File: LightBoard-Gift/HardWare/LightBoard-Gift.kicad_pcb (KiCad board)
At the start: 2 copper layers, 87.4 x 59.4 mm, 12 parts, among them SW1 SW_Push

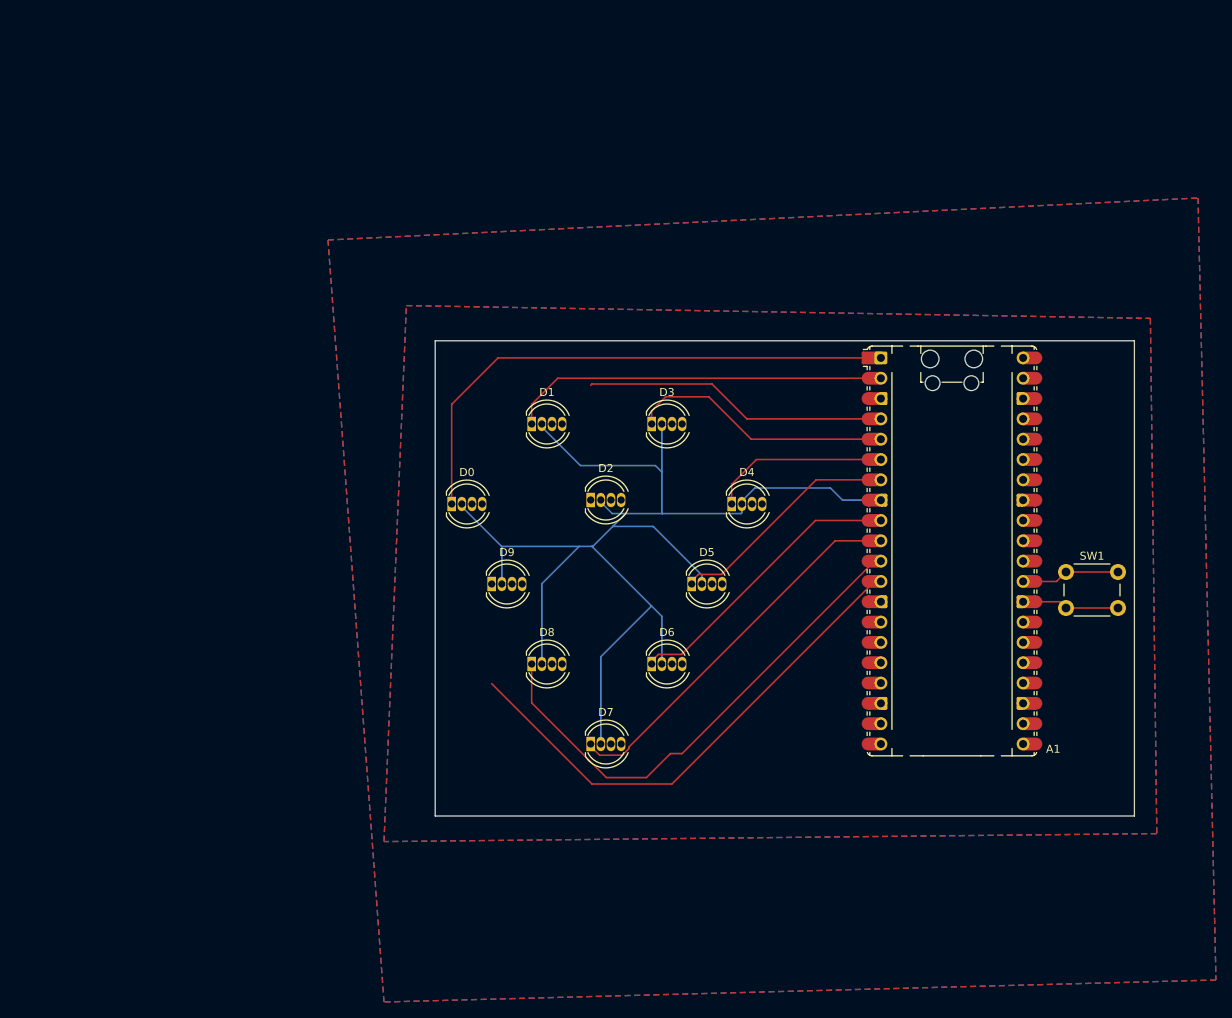
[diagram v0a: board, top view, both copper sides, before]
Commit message: Lowkey?
Forgot to save the files before pushing the last commit
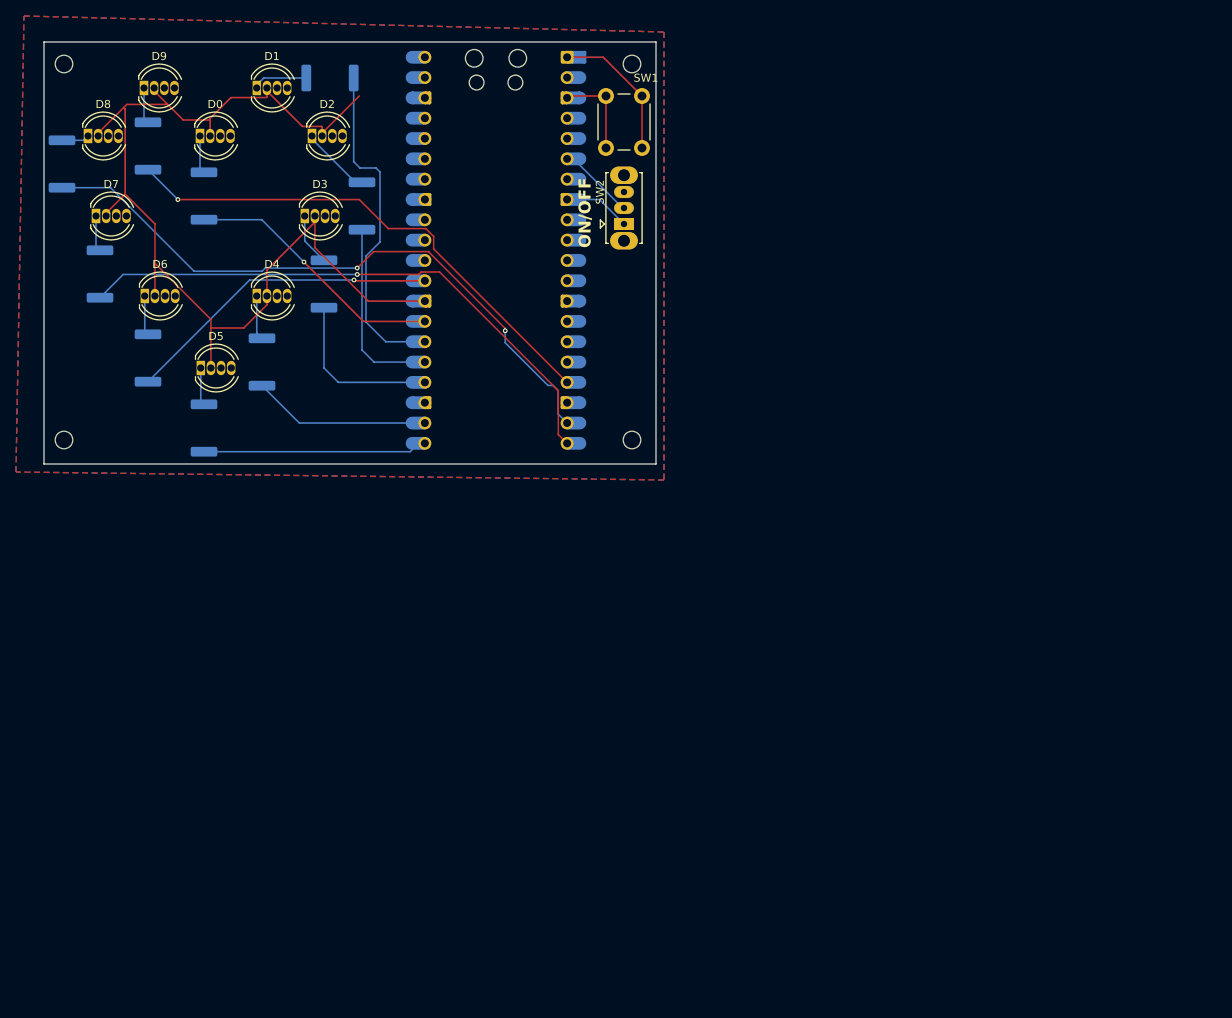
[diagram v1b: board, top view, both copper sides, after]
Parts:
- added H1: MountingHole, MountingHole:MountingHole_2.2mm_M2, F.Cu at (79.0, 25.0)
- added H2: MountingHole, MountingHole:MountingHole_2.2mm_M2, F.Cu at (79.0, 72.0)
- added H3: MountingHole, MountingHole:MountingHole_2.2mm_M2, F.Cu at (150.0, 72.0)
- added H4: MountingHole, MountingHole:MountingHole_2.2mm_M2, F.Cu at (150.0, 25.0)
- added R0: 560Ohm, Resistor_SMD:R_2512_6332Metric, B.Cu at (96.5, 41.5)
- added R1: 560Ohm, Resistor_SMD:R_2512_6332Metric, B.Cu at (112.2, 26.8)
- added R2: 560Ohm, Resistor_SMD:R_2512_6332Metric, B.Cu at (116.2, 42.8)
- added R3: R_Small, Resistor_SMD:R_2512_6332Metric, B.Cu at (111.5, 52.5)
- added R4: 560Ohm, Resistor_SMD:R_2512_6332Metric, B.Cu at (103.8, 62.2)
- added R5: 560Ohm, Resistor_SMD:R_2512_6332Metric, B.Cu at (96.5, 70.5)
- added R6: 560Ohm, Resistor_SMD:R_2512_6332Metric, B.Cu at (89.5, 61.8)
- added R7: 560Ohm, Resistor_SMD:R_2512_6332Metric, B.Cu at (83.5, 51.2)
- added R8: 560Ohm, Resistor_SMD:R_2512_6332Metric, B.Cu at (89.5, 35.2)
- added R9: 560Ohm, Resistor_SMD:R_2512_6332Metric, B.Cu at (78.8, 37.5)
- added SW2: SWITCH, Button_Switch_THT:SW_Slide_SPDT_Straight_CK_OS102011MS2Q, F.Cu at (149.0, 45.0)
- A1: moved to B.Cu
- SW1: value SW_Push -> MODE_SELECT
- moved D7 90.4 mm to (83.0, 44.0)
- moved D8 86.2 mm to (82.0, 34.0)
- moved SW1 79.7 mm to (151.2, 29.0), turned to -90 degrees
- moved D6 78.3 mm to (89.1, 54.0)
- moved D9 75.7 mm to (89.0, 28.0)
- moved A1 68.3 mm to (133.0, 48.3), turned to 180 degrees
- moved D5 67.0 mm to (96.1, 63.0)
- moved D4 64.8 mm to (103.1, 54.0)
- moved D2 57.3 mm to (110.0, 34.0)
- moved D0 55.7 mm to (96.0, 34.0)
- moved D1 54.3 mm to (103.1, 28.0)
- moved D3 50.6 mm to (109.1, 44.0)
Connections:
- A1 pad 1: RED0 -> Net-(A1-GPIO0)
- A1 pad 10: RED7 -> unconnected-(A1-GPIO7-Pad10)
- A1 pad 11: RED8 -> unconnected-(A1-GPIO8-Pad11)
- A1 pad 12: RED9 -> unconnected-(A1-GPIO9-Pad12)
- A1 pad 17: unconnected-(A1-GPIO13-Pad17) -> RED9
- A1 pad 19: unconnected-(A1-GPIO14-Pad19) -> RED8
- A1 pad 2: RED1 -> unconnected-(A1-GPIO1-Pad2)
- A1 pad 20: unconnected-(A1-GPIO15-Pad20) -> RED7
- A1 pad 21: unconnected-(A1-GPIO16-Pad21) -> RED5
- A1 pad 22: unconnected-(A1-GPIO17-Pad22) -> RED4
- A1 pad 24: unconnected-(A1-GPIO18-Pad24) -> RED3
- A1 pad 25: unconnected-(A1-GPIO19-Pad25) -> RED2
- A1 pad 26: unconnected-(A1-GPIO20-Pad26) -> RED1
- A1 pad 27: unconnected-(A1-GPIO21-Pad27) -> RED0
- A1 pad 29: Net-(A1-GPIO22) -> RED6
- A1 pad 4: RED2 -> unconnected-(A1-GPIO2-Pad4)
- A1 pad 5: RED3 -> unconnected-(A1-GPIO3-Pad5)
- A1 pad 6: RED4 -> Net-(A1-GPIO4)
- A1 pad 7: RED5 -> unconnected-(A1-GPIO5-Pad7)
- A1 pad 9: RED6 -> unconnected-(A1-GPIO6-Pad9)
- D0 pad 1: RED0 -> Net-(D0-RA)
- D1 pad 1: RED1 -> Net-(D1-RA)
- D2 pad 1: RED2 -> Net-(D2-RA)
- D3 pad 1: RED3 -> Net-(D3-RA)
- D4 pad 1: RED4 -> Net-(D4-RA)
- D5 pad 1: RED5 -> Net-(D5-RA)
- D6 pad 1: RED6 -> Net-(D6-RA)
- D7 pad 1: RED7 -> Net-(D7-RA)
- D8 pad 1: RED8 -> Net-(D8-RA)
- D9 pad 1: RED9 -> Net-(D9-RA)
- SW1 pad 1: Net-(A1-GPIO22) -> Net-(A1-GPIO0)
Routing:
- net RED0: track 67.7 -> 32.9 mm, vias 0 -> 1
- net GND: track 178.7 -> 154.6 mm
- net RED7: track 47.7 -> 71.8 mm, vias 0 -> 1
- net Net-(A1-GPIO0): track 0.00 -> 17.9 mm
- net RED8: track 62.8 -> 80.2 mm, vias 0 -> 2
- net RED2: track 37.4 -> 22.7 mm
- net RED3: track 32.7 -> 20.1 mm
- net Net-(A1-GPIO22): track 11.5 -> 0.00 mm
- net Net-(D2-RA): track 0.00 -> 8.86 mm
- net Net-(A1-GPIO4): track 0.00 -> 8.85 mm
- net Net-(D1-RA): track 0.00 -> 6.92 mm
- net Net-(D3-RA): track 0.00 -> 6.53 mm
- net Net-(D4-RA): track 0.00 -> 5.56 mm
- net RED1: track 46.7 -> 41.3 mm
- net Net-(D6-RA): track 0.00 -> 4.96 mm
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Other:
- board size 87.4 x 59.4 mm -> 76.5 x 52.8 mm
- board text added: "ON/OFF"

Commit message: Additional changes
Also fixed the function of the on/off switch
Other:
- board text added: "https://github.com/SaltyMelonYT"
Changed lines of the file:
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@@
+		)
+	)
+	(gr_text "https://github.com/SaltyMelonYT"
+		(at 128 69.627395 75)
+		(layer "B.SilkS")
+		(effects
+			(font
+				(size 1.5 1.5)
+				(thickness 0.3)
+				(bold yes)
+			)
+			(justify left bottom)
 		)
 	)
